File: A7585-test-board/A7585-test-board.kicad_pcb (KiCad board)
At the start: 4 copper layers, 82.6 x 101.6 mm, 38 parts, among them J1 Conn_01x04_Female, J100 Conn_Coaxial_Power, J2 Conn_01x20, J200 Conn_01x01_Female, J201 Conn_01x01_Female, J3 Conn_01x20, SW201 SW_SPDT, SW301 Rotary Encoder PCB, SW302 SW_Push_SPDT, SW303 SW_Push_SPDT, U100 MPM3610, U200 A7585D, U300 Pico, U301 LM4040LP-3

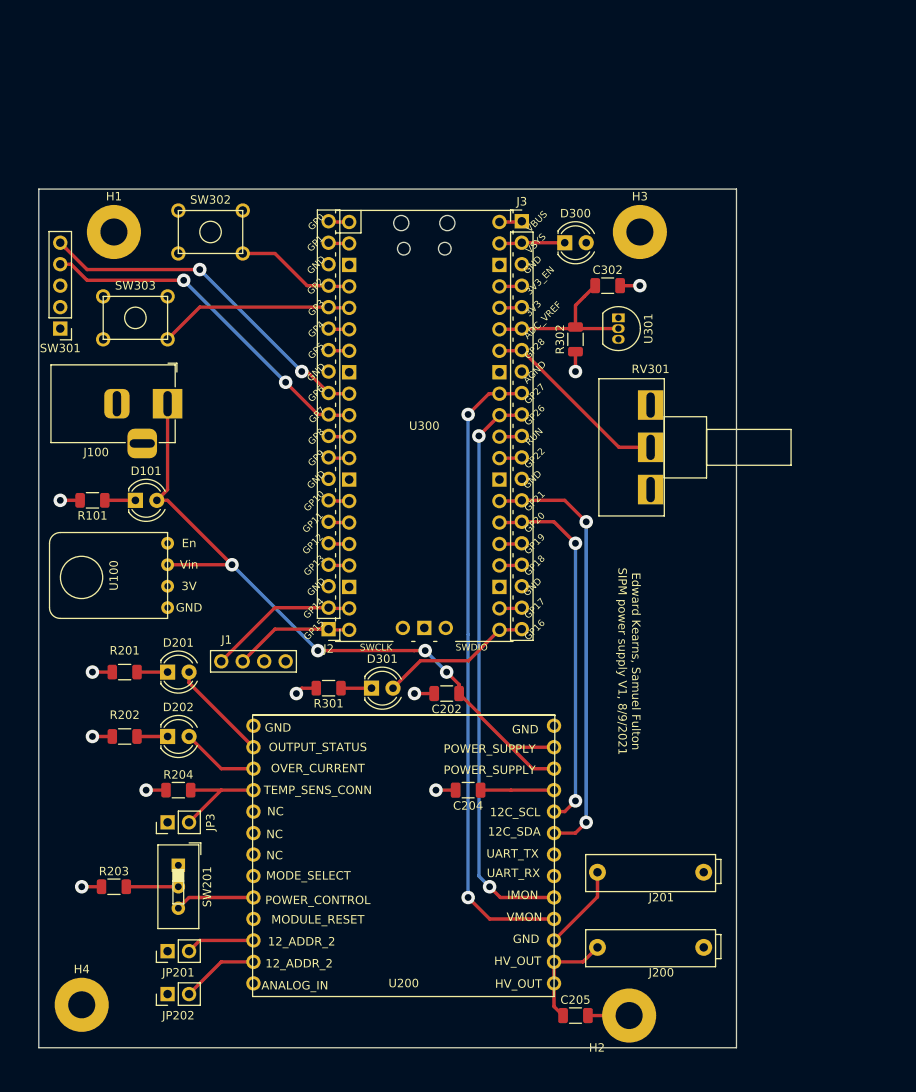
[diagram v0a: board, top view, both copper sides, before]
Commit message: Final Updates
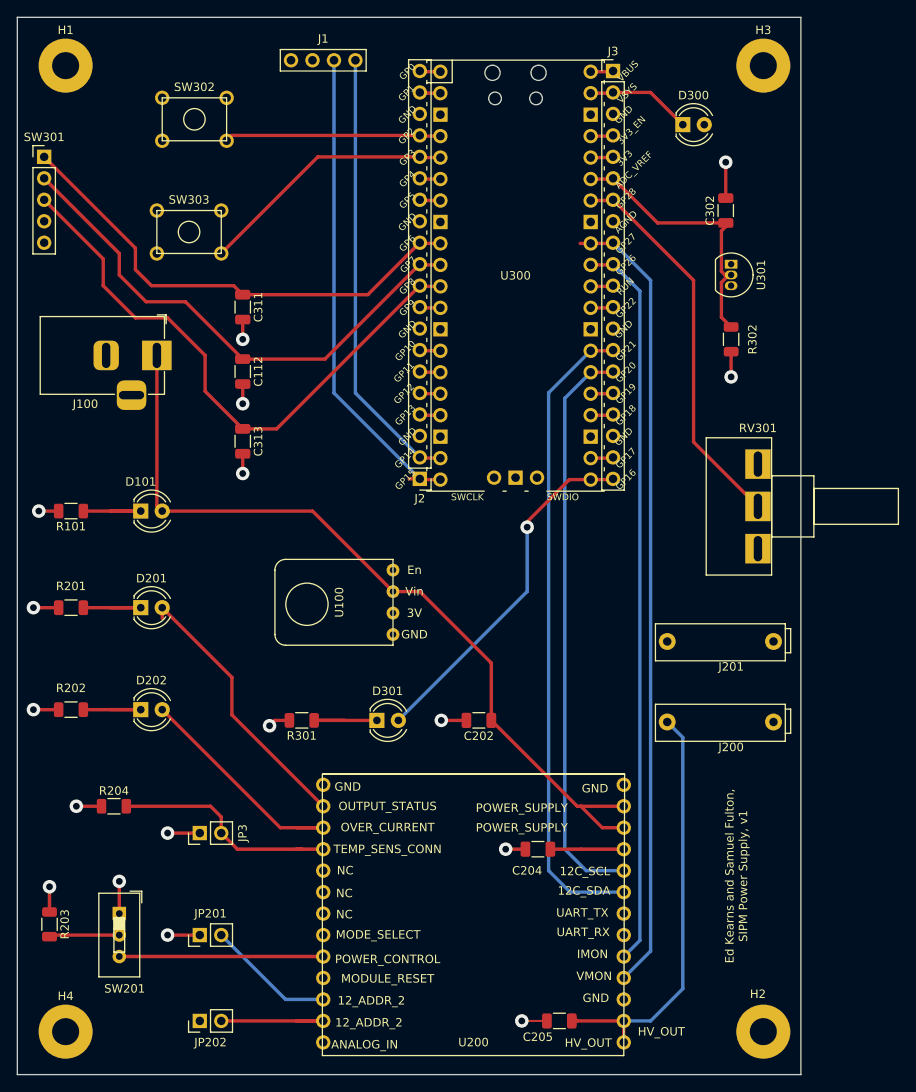
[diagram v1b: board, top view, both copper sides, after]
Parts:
- added C112: 4.7 nF, Capacitor_SMD:C_1206_3216Metric, F.Cu at (87.6, 77.5)
- added C311: 4.7 nF, Capacitor_SMD:C_1206_3216Metric, F.Cu at (87.6, 69.8)
- added C313: 4.7 nF, Capacitor_SMD:C_1206_3216Metric, F.Cu at (87.6, 85.7)
- J1: footprint A7585-test-board:Connector_Strip -> A7585-footprints:Connector_Strip
- J200, J201: footprint A7585-test-board:Bannana_Jack_2pin -> A7585-footprints:Bannana_Jack_2pin
- RV301: footprint A7585-test-board:Potentiometer_Piher_T-16H_Single_Horizontal -> A7585-footprints:Potentiometer_Piher_T-16H_Single_Horizontal
- SW201: footprint A7585-test-board:SW_DIP_SPSTx01_Slide_9.78x4.72mm_W7.62mm_P2.54mm -> A7585-footprints:SW_DIP_SPSTx01_Slide_9.78x4.72mm_W7.62mm_P2.54mm
- SW302, SW303: footprint A7585-test-board:PUSH_BUTTON -> A7585-footprints:Push_Button
- U100: footprint A7585-test-board:MPM3610 -> A7585-footprints:MPM3610
- U200: footprint A7585-test-board:A7585D_Board -> A7585-footprints:A7585D_Board
- U300: footprint A7585-test-board:RPi_Pico_SMD_TH -> A7585-footprints:RPi_Pico_SMD_TH
- moved J1 71.9 mm to (98.4, 40.6), turned to 0 degrees
- moved J201 28.5 mm to (145.4, 109.9)
- moved J200 27.9 mm to (145.4, 119.4)
- moved U100 26.9 mm to (100.3, 103.5)
- moved H3 24.5 mm to (149.2, 41.3)
- moved U300 20.8 mm to (119.9, 66.1)
- moved J2 20.8 mm to (108.6, 90.2)
- moved J3 20.8 mm to (131.4, 41.9)
- moved H1 20.5 mm to (66.7, 41.3)
- moved SW301 20.4 mm to (64.1, 52.1), turned to 0 degrees
- moved D300 19.8 mm to (139.7, 48.3)
- moved R302 18.4 mm to (145.4, 73.7)
- moved C302 16.6 mm to (144.8, 58.4), turned to 90 degrees
- moved H2 16.0 mm to (149.2, 155.6)
- moved U301 14.8 mm to (145.4, 64.8)
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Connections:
- J2 pad 10: Net-(J2-Pad10) -> Net-(C313-Pad1)
- SW301 pad 3: Net-(SW301-Pad3) -> Net-(C313-Pad1)
- U300 pad 11: Net-(J2-Pad10) -> Net-(C313-Pad1)
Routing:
- net Net-(C313-Pad1): track 0.00 -> 69.5 mm
- net Net-(J1-Pad3): track 15.5 -> 57.5 mm
- net Net-(C205-Pad1): track 12.6 -> 49.8 mm
- net Net-(J1-Pad4): track 17.8 -> 52.6 mm
- net Net-(J3-Pad14): track 51.2 -> 76.2 mm, vias 2 -> 0
- net Net-(J3-Pad15): track 43.6 -> 68.4 mm, vias 2 -> 0
- net Net-(J3-Pad7): track 22.8 -> 46.2 mm
- net Net-(D301-Pad2): track 18.1 -> 41.4 mm, vias 0 -> 1
- net Net-(D201-Pad2): track 12.0 -> 32.7 mm
- net Net-(C112-Pad1): track 41.6 -> 61.9 mm, vias 2 -> 0
- net Net-(D202-Pad2): track 9.20 -> 28.6 mm
- net Net-(J3-Pad10): track 68.2 -> 86.7 mm, vias 2 -> 0
- net Net-(J3-Pad9): track 75.8 -> 94.1 mm, vias 2 -> 0
- net Net-(C311-Pad1): track 41.6 -> 57.7 mm, vias 2 -> 0
- net Net-(JP3-Pad2): track 12.8 -> 27.8 mm
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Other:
- board size 82.6 x 101.6 mm -> 92.7 x 125.1 mm
- board text added: "Ed Kearns and Samuel Fulton, SIPM Power Supply, v1"
- board text removed: "Edward Kearns, Samuel Fulton SIPM power supply V1, 8/9/2021"
